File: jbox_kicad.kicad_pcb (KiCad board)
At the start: 2 copper layers, 52.1 x 81.3 mm, 14 parts, among them U2 mini_esp32, U3 AMS1117-3.3

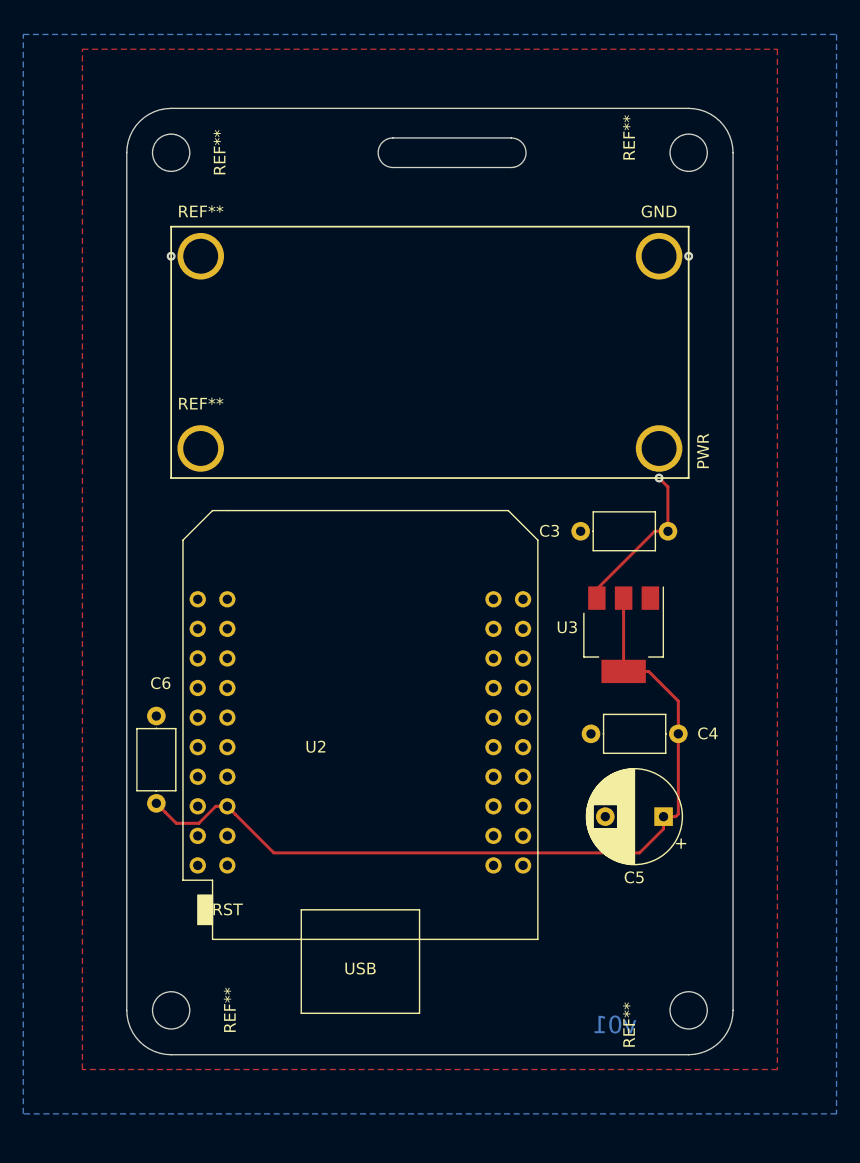
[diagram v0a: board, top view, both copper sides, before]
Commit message: 2nd version
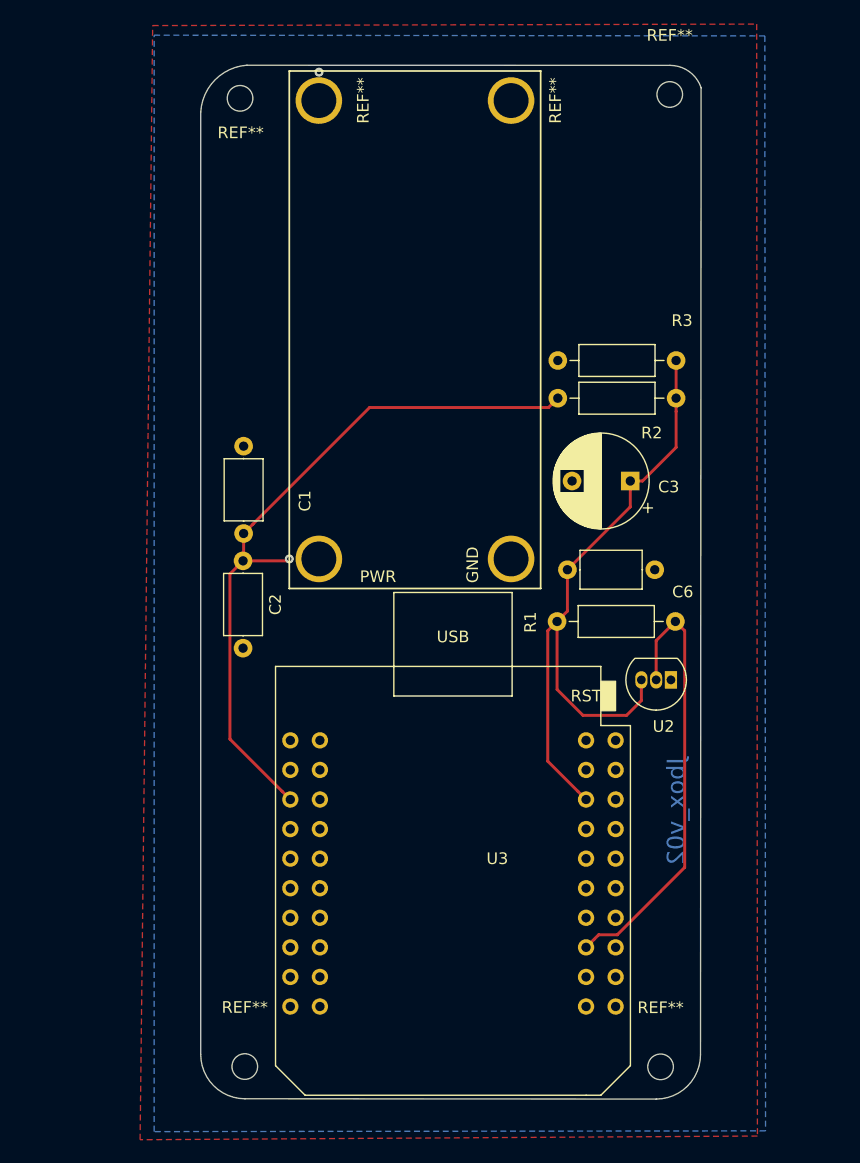
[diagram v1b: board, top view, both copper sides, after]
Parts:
- removed C4: 0.1uF, Capacitor_THT:C_Axial_L5.1mm_D3.1mm_P7.50mm_Horizontal
- removed C5: 22uF, Capacitor_THT:CP_Radial_D8.0mm_P5.00mm
- removed the REF** at (166.4, 106.7)
- removed the REF** at (166.4, 90.2)
- removed the REF** at (163.8, 154.9)
- removed the REF** at (163.8, 81.3)
- removed the REF** at (208.3, 81.3)
- removed the REF** at (208.3, 154.9)
- added C1: 100uF, Capacitor_THT:C_Axial_L5.1mm_D3.1mm_P7.50mm_Horizontal, F.Cu at (170.1, 114.0)
- added C2: 10uF, Capacitor_THT:C_Axial_L5.1mm_D3.1mm_P7.50mm_Horizontal, F.Cu at (170.0, 116.3)
- added R1: 4.7k, Resistor_THT:R_Axial_DIN0207_L6.3mm_D2.5mm_P10.16mm_Horizontal, F.Cu at (207.1, 121.5)
- added R2: 1000, Resistor_THT:R_Axial_DIN0207_L6.3mm_D2.5mm_P10.16mm_Horizontal, F.Cu at (197.0, 102.4)
- added R3: 2000, Resistor_THT:R_Axial_DIN0207_L6.3mm_D2.5mm_P10.16mm_Horizontal, F.Cu at (207.2, 99.1)
- added REF**: MountingHole_2.2mm_M2, MountingHole:MountingHole_2.2mm_M2, F.Cu at (170.2, 159.8)
- added REF**: MountingHole_2.2mm_M2, MountingHole:MountingHole_2.2mm_M2, F.Cu at (169.7, 76.6)
- added REF**: MountingHole_2.2mm_M2, MountingHole:MountingHole_2.2mm_M2, F.Cu at (205.9, 159.8)
- added REF**: MountingHole_2.2mm_M2, MountingHole:MountingHole_2.2mm_M2, F.Cu at (206.7, 76.3)
- added REF**: SolderWirePad_1x01_Drill1.5mm, Connector_Wire:SolderWirePad_1x01_Drill1.5mm, F.Cu at (176.5, 76.8)
- added REF**: SolderWirePad_1x01_Drill1.5mm, Connector_Wire:SolderWirePad_1x01_Drill1.5mm, F.Cu at (193.0, 76.8)
- C3: value 0.1uF -> 22uF; footprint Capacitor_THT:C_Axial_L5.1mm_D3.1mm_P7.50mm_Horizontal -> Capacitor_THT:CP_Radial_D8.0mm_P5.00mm
- U2: value mini_esp32 -> DS18B20; footprint ESP32_mini:ESP32_mini -> Package_TO_SOT_THT:TO-92_Inline
- U3: value AMS1117-3.3 -> mini_esp32; footprint Package_TO_SOT_SMD:SOT-223-3_TabPin2 -> ESP32_mini:ESP32_mini
- moved C6 40.6 mm to (197.9, 117.1), turned to 0 degrees
- moved PWR 30.7 mm to (176.5, 116.2), turned to 0 degrees
- moved GND 28.9 mm to (193.0, 116.2), turned to 270 degrees
- moved U2 27.0 mm to (206.8, 126.6), turned to 180 degrees
- moved U3 25.2 mm to (188.0, 143.2), turned to 180 degrees
- moved C3 5.40 mm to (203.3, 109.5)
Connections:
- C3 pad 1: /C1to1 -> VDD33
- C3 pad 2: EXT5V -> GND
- C6 pad 2: EXT5V -> GND
- GND pad 1: EXT5V -> GND
- U2 pad 1: EXT5V -> GND
- U2 pad 2: Net-(U2-Pad2) -> DQA0
- U2 pad 3: Net-(U2-Pad3) -> VDD33
- U3 pad 1: EXT5V -> GND
- U3 pad 2: VDD33 -> Net-(U3-Pad2)
- U3 pad 3: /C1to1 -> Net-(U3-Pad3)
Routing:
- net VDD5: track 0.00 -> 61.3 mm, vias 0 -> 1
- net DQA0: track 0.00 -> 38.5 mm
- net /C1to1: track 13.8 -> 0.00 mm, vias 1 -> 0
- net VDD33: track 72.2 -> 60.7 mm
- net EXT5V: track 0.19 -> 0.00 mm, vias 2 -> 0
- net VDD41: vias 0 -> 1
- added copper zone on B.Cu, net GND
- added copper zone on F.Cu, net GND
- removed copper zone on B.Cu, net EXT5V
- removed copper zone on F.Cu, net EXT5V
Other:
- board size 52.1 x 81.3 mm -> 43 x 88.8 mm
- net class Default: clearance 0.254 -> 0.199
- net class GND: clearance 0.254 -> 0.199
- rule trace_clearance: 0.254 -> 0.199
- board text added: "Jbox_v02"
- board text added: "Junction Box"
- board text removed: "v01"
